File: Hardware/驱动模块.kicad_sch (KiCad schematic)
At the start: 6 parts, among them J2 Conn_01x02_Socket, J3 Conn_01x02_Socket, J4 Conn_01x02_Socket, J5 Conn_01x02_Socket, U10 TB6612FNG, U9 TB6612FNG

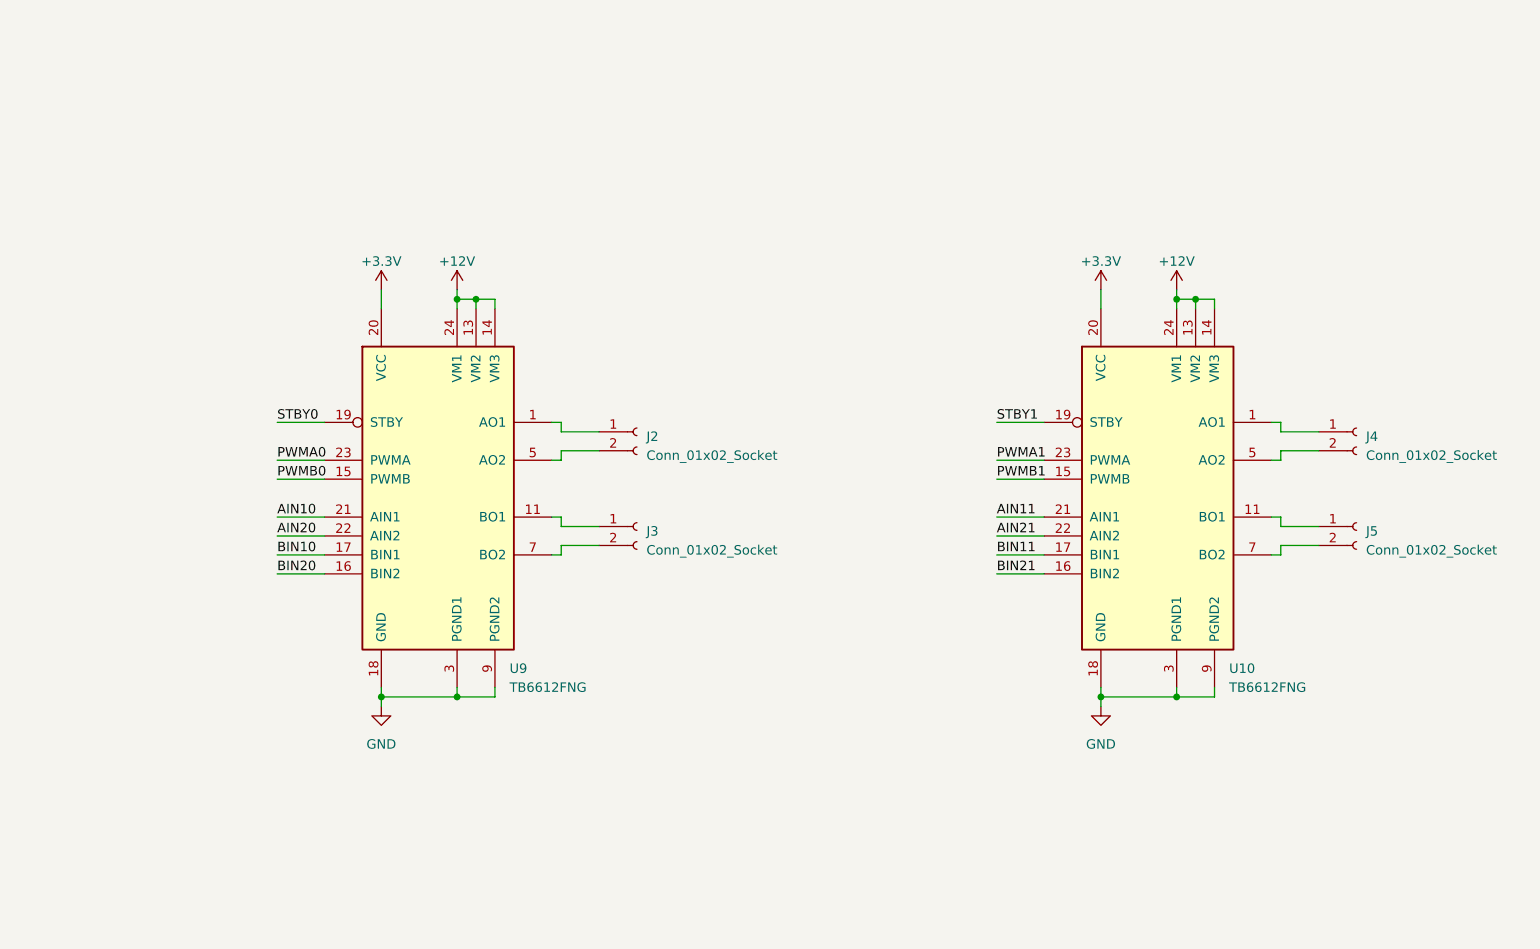
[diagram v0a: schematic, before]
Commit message: 2023/3/29
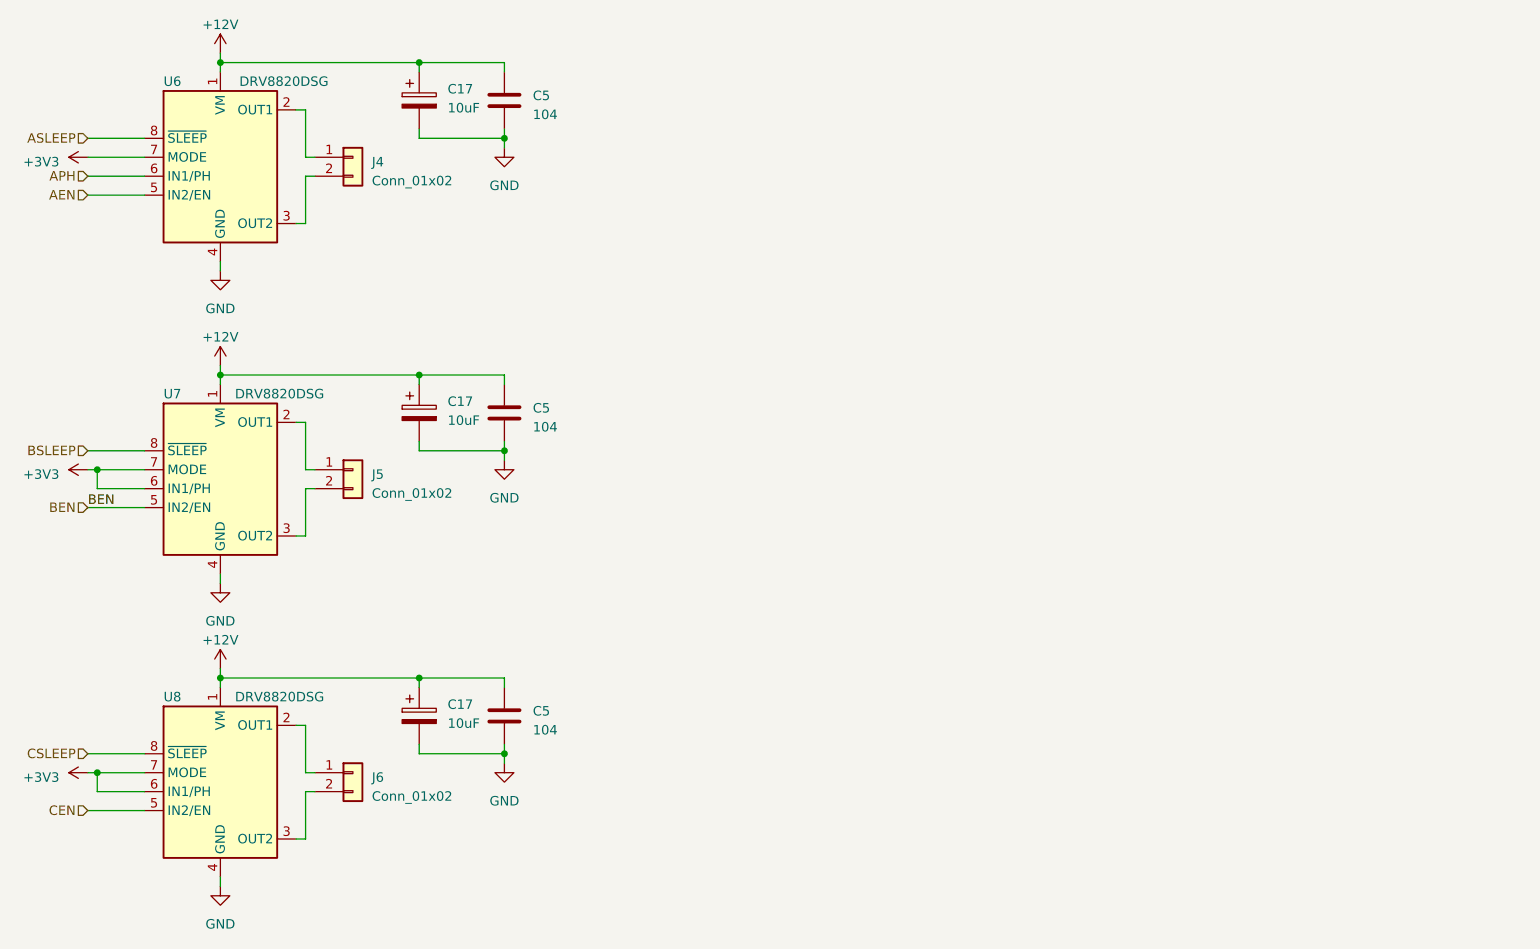
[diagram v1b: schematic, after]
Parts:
- removed J2, J3, J4, J5: Conn_01x02_Socket, symbol Connector:Conn_01x02_Socket
- removed U10, U9: TB6612FNG, Package_SO:SSOP-24_5.3x8.2mm_P0.65mm, symbol Driver_Motor:TB6612FNG
- added C17 (x3): 10uF, Capacitor_SMD:CP_Elec_4x5.4, symbol Device:C_Polarized
- added C5 (x3): 104, Capacitor_SMD:C_0402_1005Metric, symbol Device:C
- added J4, J5, J6: Conn_01x02, Connector_JST:JST_XH_B1B-XH-AM_1x01_P2.50mm_Vertical, symbol Connector_Generic:Conn_01x02
- added U6, U7, U8: DRV8820DSG, Package_SON:WSON-8-1EP_2x2mm_P0.5mm_EP0.9x1.6mm, symbol Driver_Motor:DRV8220DSG
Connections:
- net +12V: now also C17.1, C17.1, C17.1, C5.1, C5.1, C5.1, U6.1 (VM), U7.1 (VM), U8.1 (VM)
- net GND: now also C17.2, C17.2, C17.2, C5.2, C5.2, C5.2, U6.4 (GND), U6.9 (GND), U7.4 (GND), U7.9 (GND), U8.4 (GND), U8.9 (GND)
- new net: J6.1 (Pin_1), U8.2 (OUT1)
- new net: J6.2 (Pin_2), U8.3 (OUT2)
- new net: J5.1 (Pin_1), U7.2 (OUT1)
- new net: J5.2 (Pin_2), U7.3 (OUT2)
- new net: J4.1 (Pin_1), U6.2 (OUT1)
- new net: J4.2 (Pin_2), U6.3 (OUT2)
- new net +3V3: U6.7 (MODE), U7.6 (IN1/PH), U7.7 (MODE), U8.6 (IN1/PH), U8.7 (MODE)
- new net AEN: U6.5 (IN2/EN)
- new net APH: U6.6 (IN1/PH)
- new net ASLEEP: U6.8 (~{SLEEP})
- new net BEN: U7.5 (IN2/EN)
- new net BSLEEP: U7.8 (~{SLEEP})
- new net CEN: U8.5 (IN2/EN)
- new net CSLEEP: U8.8 (~{SLEEP})

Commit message: nm
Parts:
- J4, J5, J6: footprint Connector_JST:JST_XH_B1B-XH-AM_1x01_P2.50mm_Vertical -> Connector_JST:JST_XH_B2B-XH-A_1x02_P2.50mm_Vertical
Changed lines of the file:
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@@
       (effects (font (size 1.27 1.27)) (justify left))
     )
-    (property "Footprint" "Connector_JST:JST_XH_B1B-XH-AM_1x01_P2.50mm_Vertical" (at 87.63 121.92 0)
+    (property "Footprint" "Connector_JST:JST_XH_B2B-XH-A_1x02_P2.50mm_Vertical" (at 87.63 121.92 0)
       (effects (font (size 1.27 1.27)) hide)
     )
@@
   (symbol (lib_id "power:GND") (at 107.95 38.1 0) (unit 1)
     (in_bom yes) (on_board yes) (dnp no) (fields_autoplaced)
-    (property "Reference" "#PWR050" (at 107.95 44.45 0)
+    (property "Reference" "#PWR047" (at 107.95 44.45 0)
       (effects (font (size 1.27 1.27)) hide)
     )
@@
       (project "Warehouse-on-STM32"
         (path "/2599b9a9-6312-402b-9c24-1e87744a4c70/99bb5e8e-3124-4586-a004-2ab84cf92f19"
-          (reference "#PWR050") (unit 1)
+          (reference "#PWR047") (unit 1)
         )
       )
@@
   (symbol (lib_id "power:GND") (at 107.95 120.65 0) (unit 1)
     (in_bom yes) (on_board yes) (dnp no) (fields_autoplaced)
-    (property "Reference" "#PWR052" (at 107.95 127 0)
+    (property "Reference" "#PWR049" (at 107.95 127 0)
       (effects (font (size 1.27 1.27)) hide)
     )
@@
       (project "Warehouse-on-STM32"
         (path "/2599b9a9-6312-402b-9c24-1e87744a4c70/99bb5e8e-3124-4586-a004-2ab84cf92f19"
-          (reference "#PWR052") (unit 1)
+          (reference "#PWR049") (unit 1)
         )
       )
@@
   (symbol (lib_id "power:GND") (at 107.95 80.01 0) (unit 1)
     (in_bom yes) (on_board yes) (dnp no) (fields_autoplaced)
-    (property "Reference" "#PWR051" (at 107.95 86.36 0)
+    (property "Reference" "#PWR048" (at 107.95 86.36 0)
       (effects (font (size 1.27 1.27)) hide)
     )
@@
       (project "Warehouse-on-STM32"
         (path "/2599b9a9-6312-402b-9c24-1e87744a4c70/99bb5e8e-3124-4586-a004-2ab84cf92f19"
-          (reference "#PWR051") (unit 1)
+          (reference "#PWR048") (unit 1)
         )
       )
@@
       (effects (font (size 1.27 1.27)) (justify left))
     )
-    (property "Footprint" "Connector_JST:JST_XH_B1B-XH-AM_1x01_P2.50mm_Vertical" (at 87.63 39.37 0)
+    (property "Footprint" "Connector_JST:JST_XH_B2B-XH-A_1x02_P2.50mm_Vertical" (at 87.63 39.37 0)
       (effects (font (size 1.27 1.27)) hide)
     )
@@
         )
         (path "/2599b9a9-6312-402b-9c24-1e87744a4c70/99bb5e8e-3124-4586-a004-2ab84cf92f19"
-          (reference "C29") (unit 1)
+          (reference "C28") (unit 1)
         )
       )
@@
   (symbol (lib_id "power:GND") (at 69.85 54.61 0) (unit 1)
     (in_bom yes) (on_board yes) (dnp no) (fields_autoplaced)
-    (property "Reference" "#PWR045" (at 69.85 60.96 0)
+    (property "Reference" "#PWR042" (at 69.85 60.96 0)
       (effects (font (size 1.27 1.27)) hide)
     )
@@
       (project "Warehouse-on-STM32"
         (path "/2599b9a9-6312-402b-9c24-1e87744a4c70/99bb5e8e-3124-4586-a004-2ab84cf92f19"
-          (reference "#PWR045") (unit 1)
+          (reference "#PWR042") (unit 1)
         )
       )
@@
   (symbol (lib_id "power:+12V") (at 69.85 67.31 0) (unit 1)
     (in_bom yes) (on_board yes) (dnp no) (fields_autoplaced)
-    (property "Reference" "#PWR046" (at 69.85 71.12 0)
+    (property "Reference" "#PWR043" (at 69.85 71.12 0)
       (effects (font (size 1.27 1.27)) hide)
     )
@@
       (project "Warehouse-on-STM32"
         (path "/2599b9a9-6312-402b-9c24-1e87744a4c70/99bb5e8e-3124-4586-a004-2ab84cf92f19"
-          (reference "#PWR046") (unit 1)
+          (reference "#PWR043") (unit 1)
         )
       )
@@
         )
         (path "/2599b9a9-6312-402b-9c24-1e87744a4c70/99bb5e8e-3124-4586-a004-2ab84cf92f19"
-          (reference "C26") (unit 1)
+          (reference "C25") (unit 1)
         )
       )
@@
         )
         (path "/2599b9a9-6312-402b-9c24-1e87744a4c70/99bb5e8e-3124-4586-a004-2ab84cf92f19"
-          (reference "#PWR043") (unit 1)
+          (reference "#PWR040") (unit 1)
         )
       )
@@
         )
         (path "/2599b9a9-6312-402b-9c24-1e87744a4c70/99bb5e8e-3124-4586-a004-2ab84cf92f19"
-          (reference "C27") (unit 1)
+          (reference "C26") (unit 1)
         )
       )
@@
         )
         (path "/2599b9a9-6312-402b-9c24-1e87744a4c70/99bb5e8e-3124-4586-a004-2ab84cf92f19"
-          (reference "C28") (unit 1)
+          (reference "C27") (unit 1)
         )
       )
@@
         )
         (path "/2599b9a9-6312-402b-9c24-1e87744a4c70/99bb5e8e-3124-4586-a004-2ab84cf92f19"
-          (reference "#PWR042") (unit 1)
+          (reference "#PWR039") (unit 1)
         )
       )
@@
         )
         (path "/2599b9a9-6312-402b-9c24-1e87744a4c70/99bb5e8e-3124-4586-a004-2ab84cf92f19"
-          (reference "C25") (unit 1)
+          (reference "C24") (unit 1)
         )
       )
@@
         )
         (path "/2599b9a9-6312-402b-9c24-1e87744a4c70/99bb5e8e-3124-4586-a004-2ab84cf92f19"
-          (reference "C30") (unit 1)
+          (reference "C29") (unit 1)
         )
       )
@@
   (symbol (lib_id "power:+12V") (at 69.85 25.4 0) (unit 1)
     (in_bom yes) (on_board yes) (dnp no) (fields_autoplaced)
-    (property "Reference" "#PWR044" (at 69.85 29.21 0)
+    (property "Reference" "#PWR041" (at 69.85 29.21 0)
       (effects (font (size 1.27 1.27)) hide)
     )
@@
       (project "Warehouse-on-STM32"
         (path "/2599b9a9-6312-402b-9c24-1e87744a4c70/99bb5e8e-3124-4586-a004-2ab84cf92f19"
+          (reference "#PWR041") (unit 1)
+        )
+      )
+    )
+  )
+  (symbol (lib_id "power:GND") (at 69.85 96.52 0) (unit 1)
+    (in_bom yes) (on_board yes) (dnp no) (fields_autoplaced)
+    (property "Reference" "#PWR044" (at 69.85 102.87 0)
+      (effects (font (size 1.27 1.27)) hide)
+    )
+    (property "Value" "GND" (at 69.85 101.6 0)
+      (effects (font (size 1.27 1.27)))
+    )
+    (property "Footprint" "" (at 69.85 96.52 0)
+      (effects (font (size 1.27 1.27)) hide)
+    )
+    (property "Datasheet" "" (at 69.85 96.52 0)
+      (effects (font (size 1.27 1.27)) hide)
+    )
+    (pin "1")
+    (instances
+      (project "Warehouse-on-STM32"
+        (path "/2599b9a9-6312-402b-9c24-1e87744a4c70/99bb5e8e-3124-4586-a004-2ab84cf92f19"
           (reference "#PWR044") (unit 1)
-        )
-      )
-    )
-  )
-  (symbol (lib_id "power:GND") (at 69.85 96.52 0) (unit 1)
-    (in_bom yes) (on_board yes) (dnp no) (fields_autoplaced)
-    (property "Reference" "#PWR047" (at 69.85 102.87 0)
-      (effects (font (size 1.27 1.27)) hide)
-    )
-    (property "Value" "GND" (at 69.85 101.6 0)
-      (effects (font (size 1.27 1.27)))
-    )
-    (property "Footprint" "" (at 69.85 96.52 0)
-      (effects (font (size 1.27 1.27)) hide)
-    )
-    (property "Datasheet" "" (at 69.85 96.52 0)
-      (effects (font (size 1.27 1.27)) hide)
-    )
-    (pin "1")
-    (instances
-      (project "Warehouse-on-STM32"
-        (path "/2599b9a9-6312-402b-9c24-1e87744a4c70/99bb5e8e-3124-4586-a004-2ab84cf92f19"
-          (reference "#PWR047") (unit 1)
         )
       )
@@
         )
         (path "/2599b9a9-6312-402b-9c24-1e87744a4c70/99bb5e8e-3124-4586-a004-2ab84cf92f19"
-          (reference "#PWR041") (unit 1)
+          (reference "#PWR038") (unit 1)
         )
       )
@@
   (symbol (lib_id "power:GND") (at 69.85 137.16 0) (unit 1)
     (in_bom yes) (on_board yes) (dnp no) (fields_autoplaced)
-    (property "Reference" "#PWR049" (at 69.85 143.51 0)
+    (property "Reference" "#PWR046" (at 69.85 143.51 0)
       (effects (font (size 1.27 1.27)) hide)
     )
@@
       (project "Warehouse-on-STM32"
         (path "/2599b9a9-6312-402b-9c24-1e87744a4c70/99bb5e8e-3124-4586-a004-2ab84cf92f19"
-          (reference "#PWR049") (unit 1)
+          (reference "#PWR046") (unit 1)
         )
       )
@@
       (effects (font (size 1.27 1.27)) (justify left))
     )
-    (property "Footprint" "Connector_JST:JST_XH_B1B-XH-AM_1x01_P2.50mm_Vertical" (at 87.63 81.28 0)
+    (property "Footprint" "Connector_JST:JST_XH_B2B-XH-A_1x02_P2.50mm_Vertical" (at 87.63 81.28 0)
       (effects (font (size 1.27 1.27)) hide)
     )
@@
   (symbol (lib_id "power:+12V") (at 69.85 107.95 0) (unit 1)
     (in_bom yes) (on_board yes) (dnp no) (fields_autoplaced)
-    (property "Reference" "#PWR048" (at 69.85 111.76 0)
+    (property "Reference" "#PWR045" (at 69.85 111.76 0)
       (effects (font (size 1.27 1.27)) hide)
     )
@@
       (project "Warehouse-on-STM32"
         (path "/2599b9a9-6312-402b-9c24-1e87744a4c70/99bb5e8e-3124-4586-a004-2ab84cf92f19"
-          (reference "#PWR048") (unit 1)
-        )
-      )
+          (reference "#PWR045") (unit 1)
+        )
+      )
